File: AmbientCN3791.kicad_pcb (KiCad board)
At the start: 2 copper layers, 59 x 35.8 mm, 55 parts, among them J1 Conn_01x02, J2 Conn_01x02, J3 Conn_01x02, J4 Conn_01x04, J5 Conn_01x04, J6 Conn_01x02, Q1 AO4813, SW1 SW_SPDT, U1 CN3791, U2 INA3221

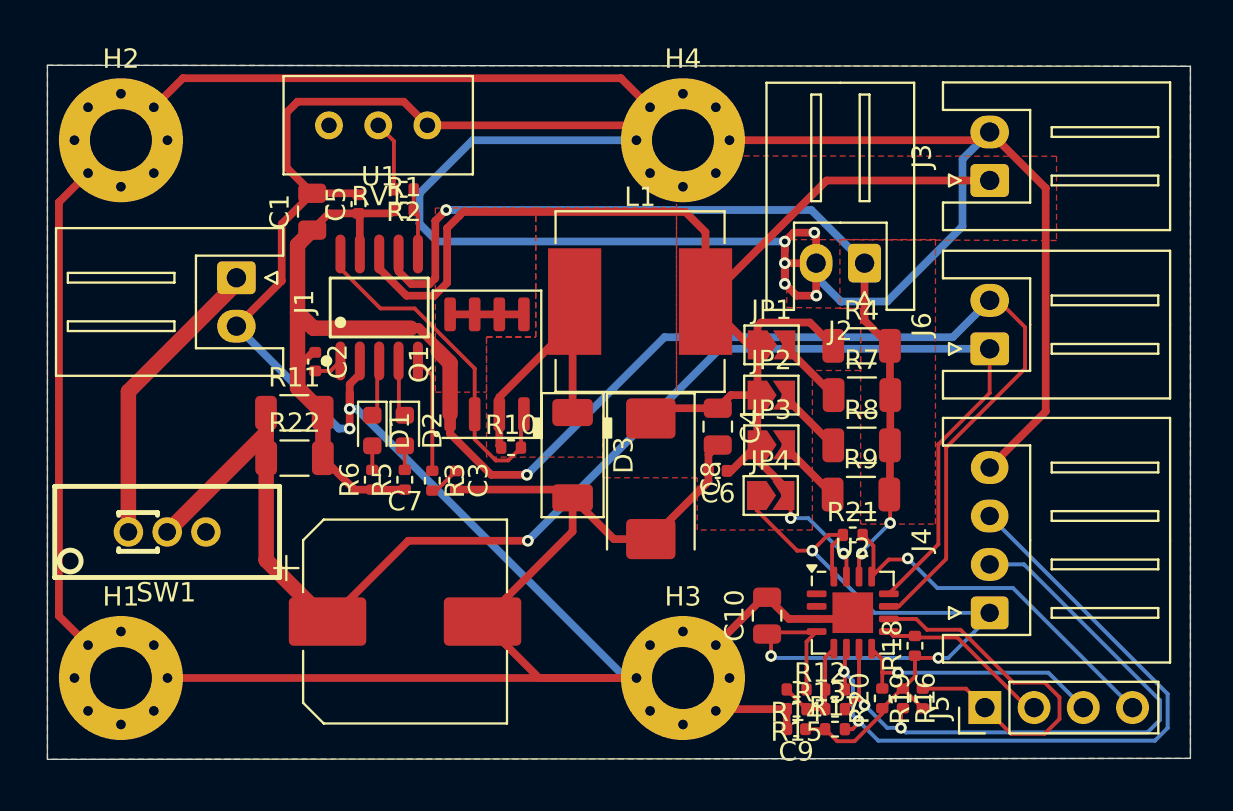
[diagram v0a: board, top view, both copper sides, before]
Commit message: AmbientCN3791 v0.1
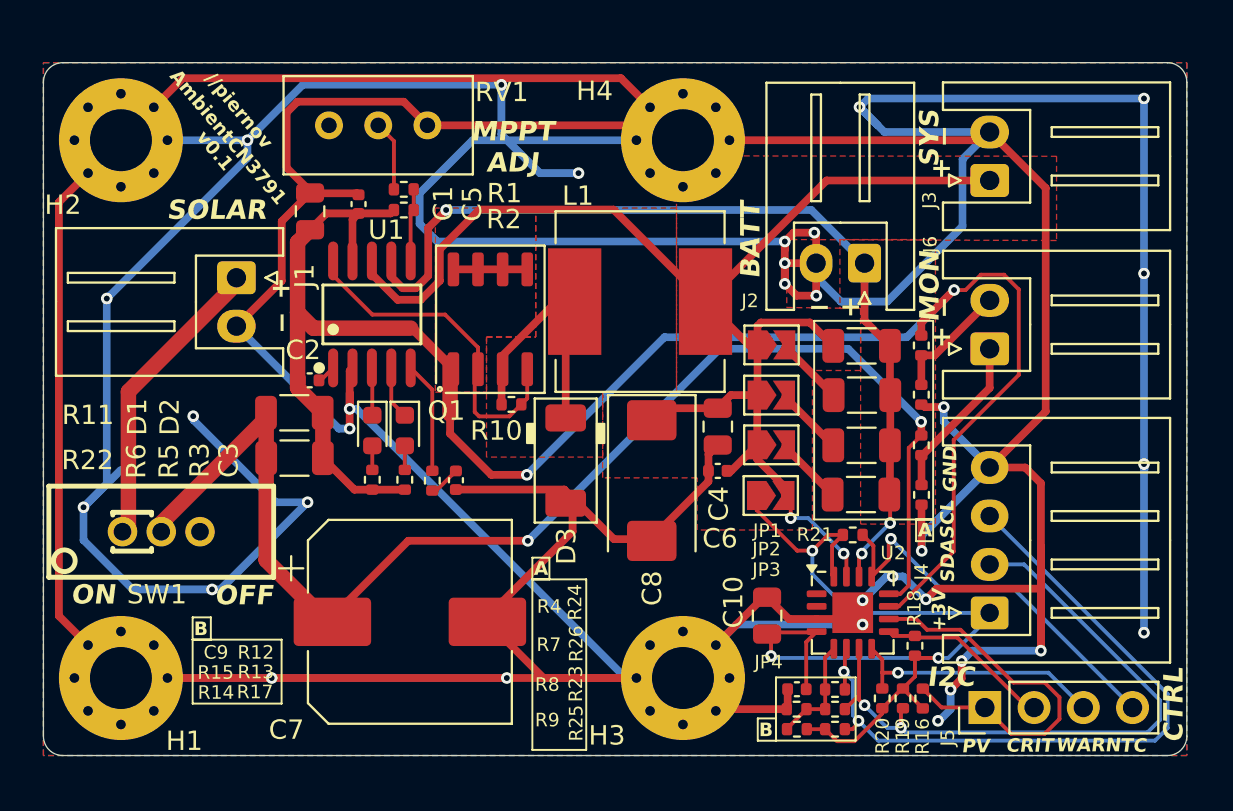
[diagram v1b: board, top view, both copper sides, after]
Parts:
- added R23: 200k, Resistor_SMD:R_0402_1005Metric, F.Cu at (150.3, 75.7)
- added R24: 200k, Resistor_SMD:R_0402_1005Metric, F.Cu at (150.3, 70.6)
- added R25: 20k, Resistor_SMD:R_0402_1005Metric, F.Cu at (150.3, 78.3)
- added R26: 20k, Resistor_SMD:R_0402_1005Metric, F.Cu at (150.3, 73.1)
- D1: value LED_Small -> KT-0603R
- D2: value LED_Small -> KT-0603W
- moved Q1 2.33 mm to (128.1, 69.2)
- moved R10 2.23 mm to (129.2, 73.6)
- moved C9 2.06 mm to (143.9, 88.3)
- moved R14 2.05 mm to (143.9, 90.4)
- moved C2 1.01 mm to (118.7, 72.4), turned to 0 degrees
- moved U1 0.52 mm to (122.0, 69.0)
- moved D3 0.45 mm to (131.9, 76.5)
- moved SW1 0.31 mm to (111.1, 80.2)
- moved C7 0.25 mm to (123.9, 84.8)
- moved C1 0.11 mm to (118.8, 63.7)
- moved C8 0.10 mm to (136.4, 77.6)
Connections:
- J6 pad 1: CSIP -> Net-(J6-Pin_1)
- J6 pad 2: CSIN -> Net-(J6-Pin_2)
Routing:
- net GND: track 318.3 -> 530.4 mm, vias 7 -> 32
- net Net-(J6-Pin_1): track 0.00 -> 9.12 mm
- net Net-(J6-Pin_2): track 0.00 -> 6.66 mm
- net CSIP: track 75.1 -> 68.6 mm, vias 1 -> 2
- net CSOP: track 74.7 -> 72.3 mm
- net Net-(D3-K): track 15.0 -> 12.9 mm
- net Net-(J5-Pin_4): track 19.6 -> 20.9 mm
- net CSIN: track 96.9 -> 98.0 mm, vias 1 -> 2
- net Net-(J4-Pin_1): track 49.9 -> 50.6 mm
- net Net-(Q1A-G1): track 18.4 -> 17.8 mm
- net Net-(U1-VG): track 1.51 -> 1.00 mm
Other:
- outline, holes or cut-outs redrawn
- board text added: "+"
- board text added: "+3V"
- board text added: "//piernov"
- board text added: "//piernov AmbientCN3791 v0.1"
- board text added: "A"
- board text added: "AmbientCN3791"
- board text added: "B"
- board text added: "BATT"
- board text added: "CRIT"
- board text added: "CTRL"
- board text added: "GND"
- board text added: "I2C"
- board text added: "MON"
- board text added: "MPPT ADJ"
- board text added: "OFF"
- board text added: "ON"
- board text added: "PV"
- board text added: "SCL"
- board text added: "SDA"
- board text added: "SOLAR"
- board text added: "SYS"
- board text added: "TC"
- board text added: "WARN"
- board text added: "v0.1"
- board text added: "−"
